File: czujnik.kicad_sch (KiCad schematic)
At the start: 8 parts, among them J6 Conn_C, U3 BME280, U6 MB85RS256B

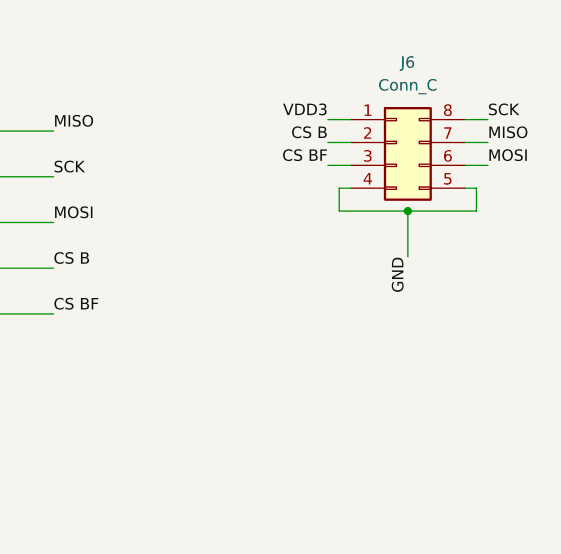
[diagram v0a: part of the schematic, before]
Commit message: Orange 21.37
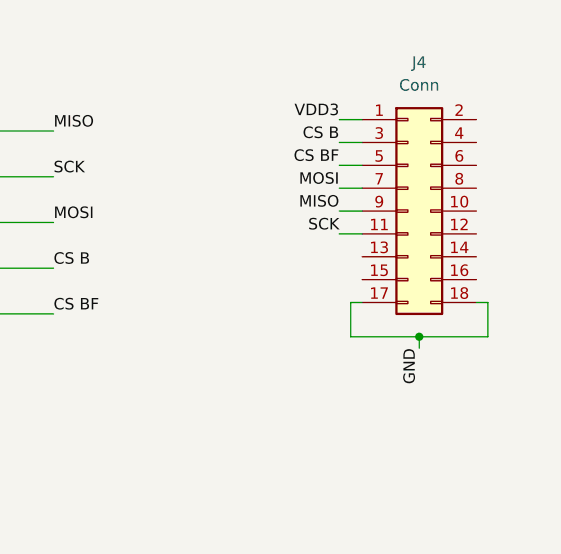
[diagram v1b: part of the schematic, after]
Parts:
- removed J6: Conn_C, symbol Connector_Generic:Conn_02x04_Counter_Clockwise
- added J4: Conn, symbol Connector_Generic:Conn_02x09_Odd_Even
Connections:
- net CS B: now also J4.3 (Pin_3)
- net CS BF: now also J4.5 (Pin_5)
- net GND: now also J4.17 (Pin_17), J4.18 (Pin_18)
- net MISO: now also J4.9 (Pin_9)
- net MOSI: now also J4.7 (Pin_7)
- net SCK: now also J4.11 (Pin_11)
- net VDD3: now also J4.1 (Pin_1)
